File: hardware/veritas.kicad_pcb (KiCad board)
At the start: 2 copper layers, 43 parts, among them J1 ~{USB_BOOT}, J2 USB_C_Receptacle_USB2.0, J3 VIDEO, J4 VIDEO, J5 SYNC, J6 CONTROLLER_PORT, J7 CON_RESET, Q1 LMBT3946DW1T1G, U1 W25Q128JVSIQ, U2 NCP1117ST33T3G, U3 RP2040, U4 LM1881, Y1 12MHz

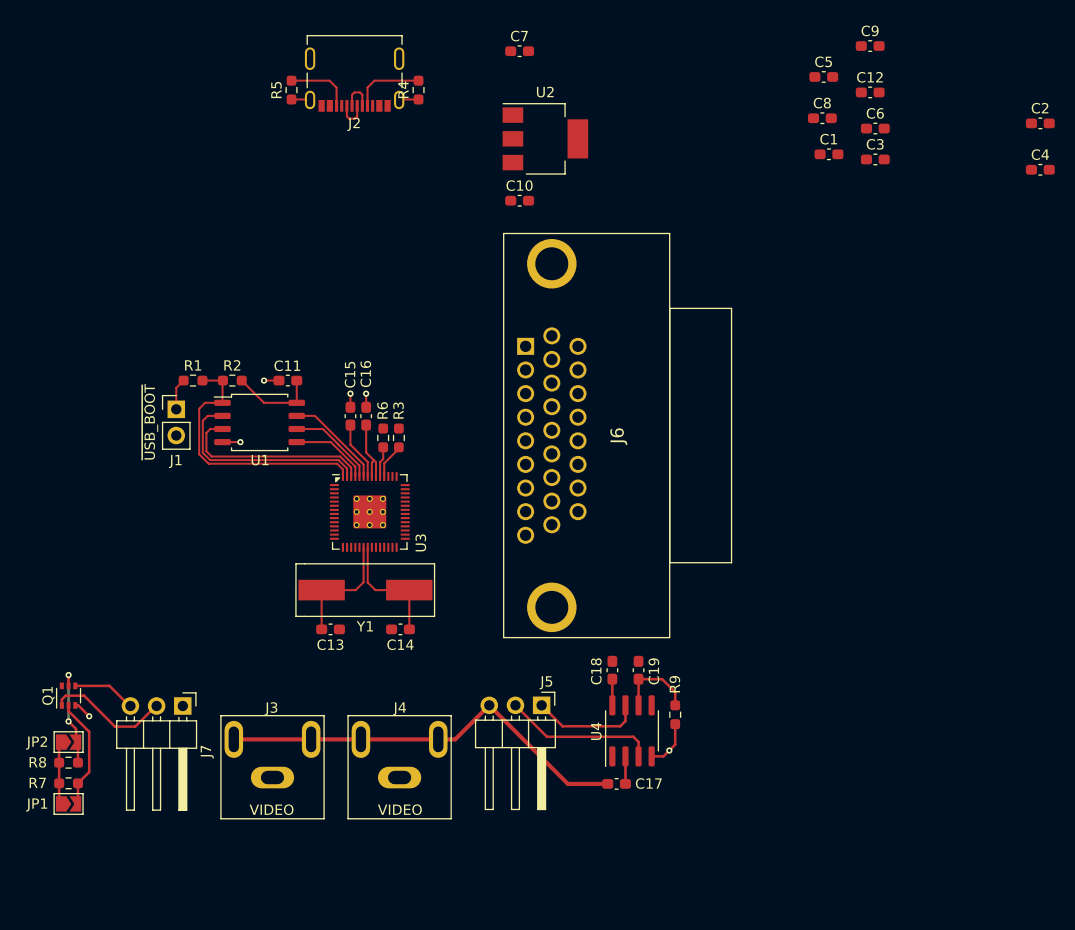
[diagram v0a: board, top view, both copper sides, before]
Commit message: Finished first hardware prototype.
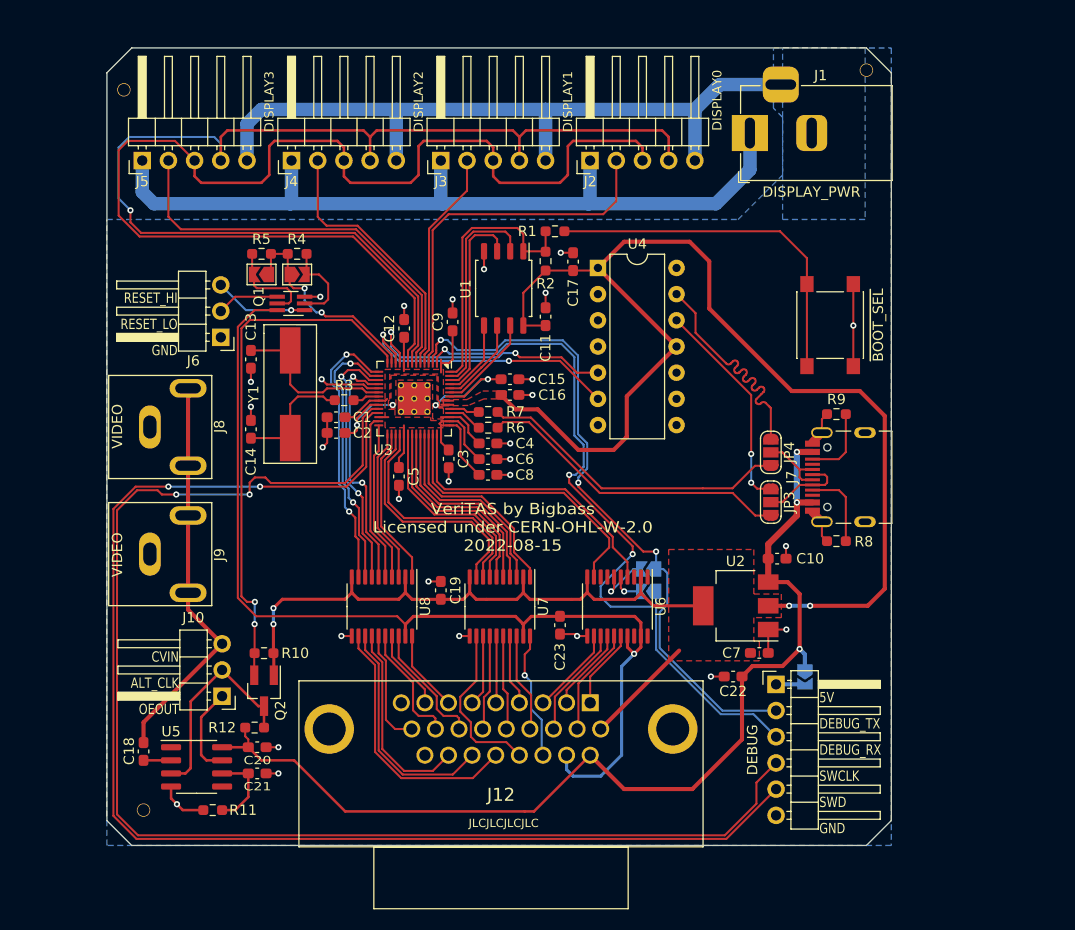
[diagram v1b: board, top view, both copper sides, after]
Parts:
- added C17: 0.1uF, Capacitor_SMD:C_0603_1608Metric_Pad1.08x0.95mm_HandSolder, F.Cu at (154.7, 79.9)
- added C19: 0.1uF, Capacitor_SMD:C_0603_1608Metric_Pad1.08x0.95mm_HandSolder, F.Cu at (141.9, 111.8)
- added C22: 0.1uF, Capacitor_SMD:C_0603_1608Metric_Pad1.08x0.95mm_HandSolder, F.Cu at (170.2, 120.1)
- added C23: 0.1uF, Capacitor_SMD:C_0603_1608Metric_Pad1.08x0.95mm_HandSolder, F.Cu at (153.4, 115.2)
- added J11: DEBUG, Connector_PinHeader_2.54mm:PinHeader_1x06_P2.54mm_Horizontal, F.Cu at (174.4, 120.9)
- added J2: DISPLAY0, Connector_PinHeader_2.54mm:PinHeader_1x05_P2.54mm_Horizontal, F.Cu at (156.3, 70.1)
- added J3: DISPLAY1, Connector_PinHeader_2.54mm:PinHeader_1x05_P2.54mm_Horizontal, F.Cu at (141.9, 70.1)
- added J4: DISPLAY2, Connector_PinHeader_2.54mm:PinHeader_1x05_P2.54mm_Horizontal, F.Cu at (127.4, 70.1)
- added J5: DISPLAY3, Connector_PinHeader_2.54mm:PinHeader_1x05_P2.54mm_Horizontal, F.Cu at (112.9, 70.1)
- added JP3: DJ-, Jumper:SolderJumper-3_P1.3mm_Open_RoundedPad1.0x1.5mm_NumberLabels, F.Cu at (173.9, 103.2)
- added JP4: DJ+, Jumper:SolderJumper-3_P1.3mm_Open_RoundedPad1.0x1.5mm_NumberLabels, F.Cu at (173.9, 98.4)
- added JP5: SolderJumper_2_Open, Jumper:SolderJumper-2_P1.3mm_Open_TrianglePad1.0x1.5mm, B.Cu at (162.0, 111.9)
- added JP6: SolderJumper_2_Open, Jumper:SolderJumper-2_P1.3mm_Open_TrianglePad1.0x1.5mm, B.Cu at (162.0, 109.7)
- added JP7: SolderJumper_2_Open, Jumper:SolderJumper-2_P1.3mm_Open_TrianglePad1.0x1.5mm, B.Cu at (177.2, 120.2)
- added Q2: 2N7002K, Package_TO_SOT_SMD:SOT-23_Handsoldering, F.Cu at (124.7, 121.5)
- added R10: 10K, Resistor_SMD:R_0603_1608Metric_Pad0.98x0.95mm_HandSolder, F.Cu at (124.7, 117.9)
- added R12: 10K, Resistor_SMD:R_0603_1608Metric_Pad0.98x0.95mm_HandSolder, F.Cu at (123.8, 125.1)
- added R3: 1K, Resistor_SMD:R_0603_1608Metric_Pad0.98x0.95mm_HandSolder, F.Cu at (132.5, 93.3)
- added REF**: JLC_ToolingHole, veritas:JLC_ToolingHole, F.Cu at (183.1, 61.3)
- added REF**: JLC_ToolingHole, veritas:JLC_ToolingHole, F.Cu at (111.1, 63.2)
- added REF**: JLC_ToolingHole, veritas:JLC_ToolingHole, F.Cu at (113.0, 133.1)
- added SW1: ~{BOOT_SEL}, Button_Switch_SMD:SW_SPST_PTS645, F.Cu at (179.6, 86.1)
- added U4: MCP2221A, Package_DIP:DIP-14_W7.62mm, F.Cu at (157.1, 80.5)
- added U6: TXS0108EPW, Package_SO:TSSOP-20_4.4x6.5mm_P0.65mm, F.Cu at (159.0, 113.4)
- added U7: TXS0108EPW, Package_SO:TSSOP-20_4.4x6.5mm_P0.65mm, F.Cu at (147.6, 113.4)
- added U8: TXS0108EPW, Package_SO:TSSOP-20_4.4x6.5mm_P0.65mm, F.Cu at (136.1, 113.4)
- J1: value ~{USB_BOOT} -> DISPLAY_PWR; footprint Connector_PinHeader_2.54mm:PinHeader_1x02_P2.54mm_Vertical -> Connector_BarrelJack:BarrelJack_Horizontal
- J7: renamed from J2; value USB_C_Receptacle_USB2.0 -> USB2.0_C; footprint veritas:2171790001 -> veritas:TYPE-C-31-M-12
- Q1: footprint Package_TO_SOT_SMD:SOT-363_SC-70-6 -> Package_TO_SOT_SMD:SOT-363_SC-70-6_Handsoldering
- moved C2 74.6 mm to (131.7, 96.5), turned to 180 degrees
- moved J7 63.2 mm to (183.0, 100.8), turned to 90 degrees
- moved C7 62.8 mm to (172.7, 117.9)
- moved J1 61.7 mm to (171.8, 67.4), turned to 180 degrees
- moved R9 61.5 mm to (180.2, 94.7), turned to 0 degrees
- moved C4 59.8 mm to (146.4, 97.5)
- moved R8 59.6 mm to (180.2, 107.0), turned to 0 degrees
- moved C5 56.6 mm to (137.8, 100.7), turned to -90 degrees
- moved JP1 55.9 mm to (127.9, 81.2)
- moved R4 55.9 mm to (127.9, 79.2)
- moved C1 54.2 mm to (131.7, 95.0), turned to 180 degrees
- moved R5 52.8 mm to (124.5, 79.2), turned to 0 degrees
- moved C12 50.7 mm to (138.3, 86.4), turned to 90 degrees
- moved C3 50.5 mm to (142.6, 99.0), turned to -90 degrees
- moved C6 49.4 mm to (146.4, 99.1)
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- renumbered C17 to C18, C18 to C20, C19 to C21, J5 to J10, J6 to J12, J7 to J6, J3 to J8, J4 to J9, R9 to R11, R7 to R4, R8 to R5, R3 to R6, R6 to R7, R4 to R8, R5 to R9, U4 to U5
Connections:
- net ALT_CLK renamed ALT_CLK_B
- J1 pad 1: Net-(J1-Pad1) -> /LED_5V
- J12 pad 1: unconnected-(J6-Pad1) -> CP_1
- J12 pad 10: VBUS -> +3V3
- J12 pad 11: unconnected-(J6-Pad11) -> CP_11
- J12 pad 12: unconnected-(J6-Pad12) -> CP_12
- J12 pad 13: unconnected-(J6-Pad13) -> CP_13
- J12 pad 14: unconnected-(J6-Pad14) -> CP_14
- J12 pad 15: unconnected-(J6-Pad15) -> CP_15
- J12 pad 16: unconnected-(J6-Pad16) -> CP_16
- J12 pad 17: unconnected-(J6-Pad17) -> CP_17
- J12 pad 18: unconnected-(J6-Pad18) -> CP_18
- J12 pad 19: +3V3 -> VBUS
- J12 pad 2: unconnected-(J6-Pad2) -> CP_2
- J12 pad 20: unconnected-(J6-Pad20) -> CP_20
- J12 pad 21: unconnected-(J6-Pad21) -> CP_21
- J12 pad 22: unconnected-(J6-Pad22) -> CP_22
- J12 pad 23: unconnected-(J6-Pad23) -> CP_23
- J12 pad 24: unconnected-(J6-Pad24) -> CP_24
- J12 pad 25: unconnected-(J6-Pad25) -> CP_25
- J12 pad 3: unconnected-(J6-Pad3) -> CP_3
- J12 pad 4: unconnected-(J6-Pad4) -> CP_4
- J12 pad 5: unconnected-(J6-Pad5) -> CP_5
- J12 pad 6: unconnected-(J6-Pad6) -> CP_6
- J12 pad 7: unconnected-(J6-Pad7) -> CP_7
- J12 pad 8: unconnected-(J6-Pad8) -> CP_8
- J6 pad 2: /RESET_HI -> /RESET_LO
- J6 pad 3: /RESET_LO -> /RESET_HI
- J7 pad A6: /D+ -> /PORTD+
- J7 pad A7: /D- -> /PORTD-
- J7 pad B6: /D+ -> /PORTD+
- J7 pad B7: /D- -> /PORTD-
- Q1 pad 6: VDD -> CP_20
- R1 pad 1: Net-(J1-Pad1) -> Net-(R1-Pad1)
- U3 pad 11: unconnected-(U3-Pad11) -> BRIDGE_RX
- U3 pad 12: unconnected-(U3-Pad12) -> BRIDGE_TX
- U3 pad 13: unconnected-(U3-Pad13) -> CON_RESET
- U3 pad 14: unconnected-(U3-Pad14) -> ALT_CLK_A
- U3 pad 15: unconnected-(U3-Pad15) -> CNT_0
- U3 pad 16: unconnected-(U3-Pad16) -> CNT_1
- U3 pad 17: unconnected-(U3-Pad17) -> CNT_2
- U3 pad 18: unconnected-(U3-Pad18) -> CNT_3
- U3 pad 19: unconnected-(U3-Pad19) -> GND
- U3 pad 2: unconnected-(U3-Pad2) -> CNT_17
- U3 pad 21: Net-(C14-Pad2) -> Net-(R3-Pad2)
- U3 pad 24: unconnected-(U3-Pad24) -> SWCLK
- U3 pad 25: unconnected-(U3-Pad25) -> SWD
- U3 pad 26: unconnected-(U3-Pad26) -> +3V3
- U3 pad 27: unconnected-(U3-Pad27) -> CNT_4
- U3 pad 28: unconnected-(U3-Pad28) -> CNT_5
- U3 pad 29: unconnected-(U3-Pad29) -> CNT_6
- U3 pad 3: unconnected-(U3-Pad3) -> CNT_18
- U3 pad 30: unconnected-(U3-Pad30) -> CNT_7
- U3 pad 31: unconnected-(U3-Pad31) -> CNT_8
- U3 pad 32: unconnected-(U3-Pad32) -> CNT_9
- U3 pad 34: unconnected-(U3-Pad34) -> CNT_10
- U3 pad 35: unconnected-(U3-Pad35) -> CNT_11
- U3 pad 36: unconnected-(U3-Pad36) -> CNT_12
- U3 pad 37: unconnected-(U3-Pad37) -> CNT_13
- U3 pad 38: unconnected-(U3-Pad38) -> CNT_14
- U3 pad 39: unconnected-(U3-Pad39) -> CNT_15
- U3 pad 4: unconnected-(U3-Pad4) -> DISPLAY_STROBE0
- U3 pad 40: unconnected-(U3-Pad40) -> CNT_16
- U3 pad 41: unconnected-(U3-Pad41) -> DETECT
- U3 pad 5: unconnected-(U3-Pad5) -> DISPLAY_STROBE1
- U3 pad 6: unconnected-(U3-Pad6) -> DISPLAY_STROBE2
- U3 pad 7: unconnected-(U3-Pad7) -> DISPLAY_STROBE3
- U3 pad 8: unconnected-(U3-Pad8) -> DISPLAY_SER
- U3 pad 9: unconnected-(U3-Pad9) -> DISPLAY_CLK
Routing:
- net +3V3: track 15.4 -> 225.7 mm, vias 0 -> 4
- net SWCLK: track 0.00 -> 132.0 mm, vias 0 -> 2
- net SWD: track 0.00 -> 129.2 mm, vias 0 -> 2
- net GND: track 16.1 -> 135.4 mm, vias 6 -> 28
- net DISPLAY_CLK: track 0.00 -> 116.8 mm
- net DISPLAY_SER: track 0.00 -> 111.7 mm, vias 0 -> 1
- net VBUS: track 2.54 -> 101.3 mm, vias 0 -> 3
- net CP_20: track 0.00 -> 97.9 mm, vias 0 -> 1
- net /LED_5V: track 0.00 -> 80.1 mm
- net CNT_17: track 0.00 -> 70.3 mm, vias 0 -> 3
- net CNT_18: track 0.00 -> 65.2 mm, vias 0 -> 3
- net ALT_CLK_A: track 0.00 -> 51.3 mm, vias 0 -> 2
- net DISPLAY_STROBE3: track 0.00 -> 40.0 mm
- net DISPLAY_STROBE0: track 0.00 -> 36.0 mm
- net Net-(R1-Pad1): track 0.00 -> 35.1 mm
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- added copper zone on F.Cu, net +1V1
- added copper zone on F.Cu, net +3V3
- added copper zone on B.Cu, net GND
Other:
- board outline added: 76.1 x 77.3 mm
- board text added: "5V"
- board text added: "ALT_CLK"
- board text added: "CVIN"
- board text added: "DEBUG_RX"
- board text added: "DEBUG_TX"
- board text added: "GND"
- board text added: "JLCJLCJLCJLC"
- board text added: "OEOUT"
- board text added: "RESET_HI"
- board text added: "RESET_LO"
- board text added: "SWCLK"
- board text added: "SWD"
- board text added: "VeriTAS by Bigbass Licensed under CERN-OHL-W-2.0 2022-08-15"
